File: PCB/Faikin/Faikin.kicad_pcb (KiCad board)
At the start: 2 copper layers, 70 x 70 mm, 27 parts, among them J1 1x5, J2 TC2030-USB-NL-DS, Q1 BSS138PS, U3 MD8942, U4 ESP32-S3-MINI-1

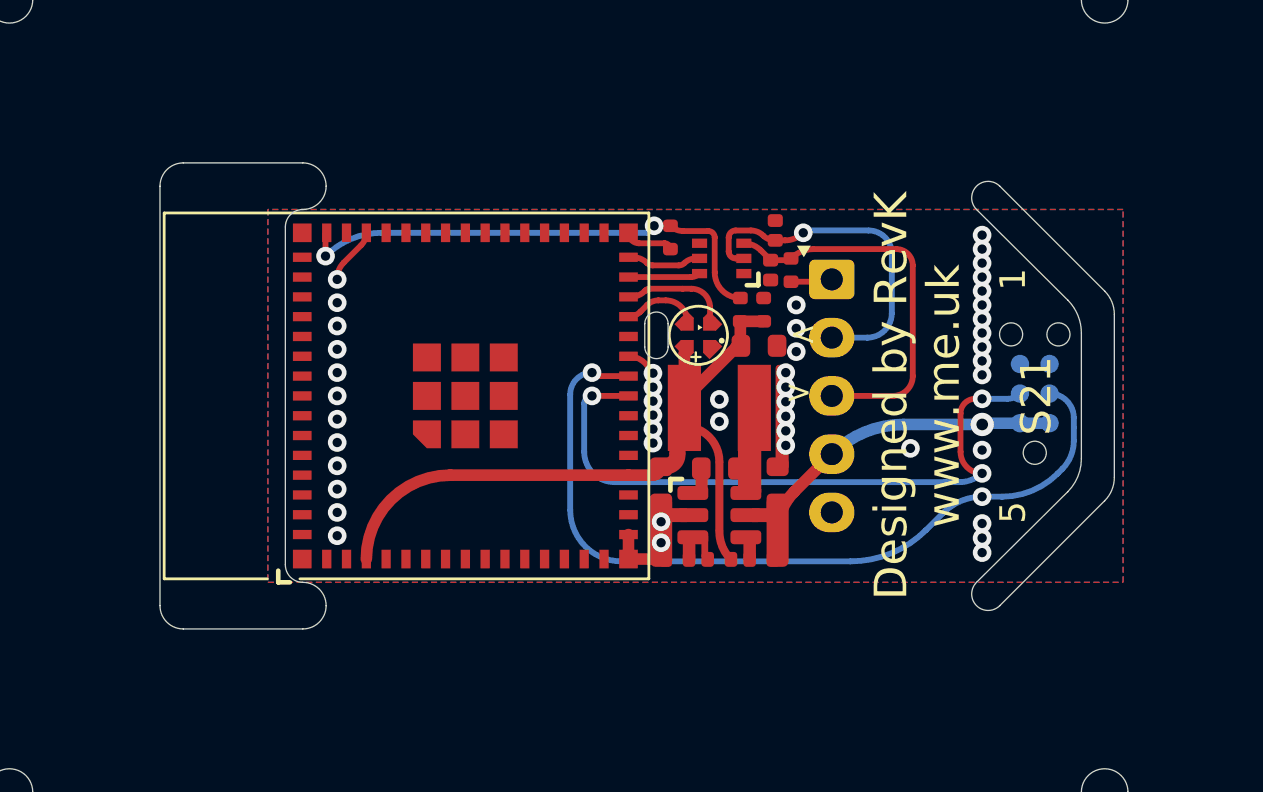
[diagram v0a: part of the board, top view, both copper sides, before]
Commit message: Origin
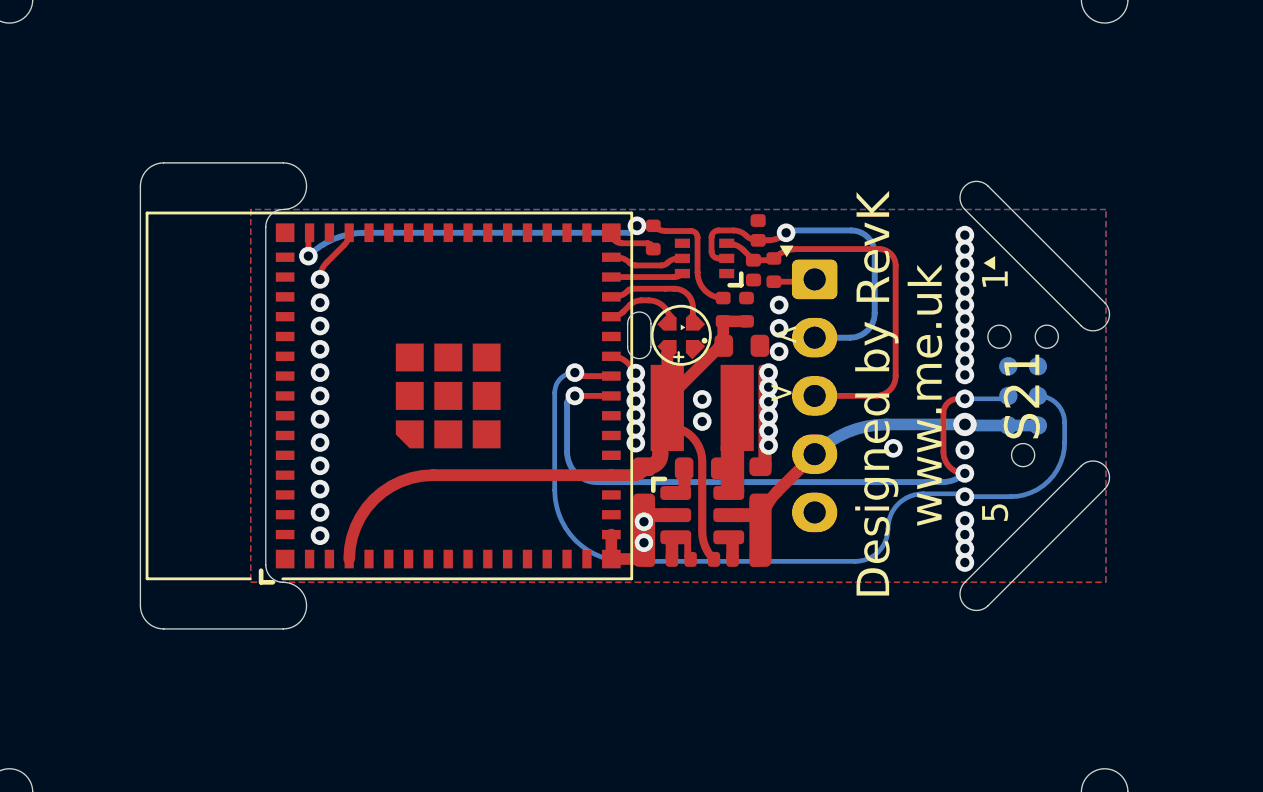
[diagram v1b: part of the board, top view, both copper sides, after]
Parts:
- moved C10 0.74 mm to (140.7, 68.1)
- moved C2 0.74 mm to (142.6, 61.3)
- moved C6 0.74 mm to (138.6, 58.2)
- moved C8 0.74 mm to (143.2, 68.8)
- moved C9 0.74 mm to (138.2, 68.8)
- moved D3 0.74 mm to (143.1, 57.9)
- moved L2 0.74 mm to (140.7, 65.5)
- moved R3 0.74 mm to (141.6, 61.3)
- moved R9 0.74 mm to (140.7, 72.0)
- moved U3 0.74 mm to (140.7, 70.1)
- moved C5 0.73 mm to (142.4, 62.9)
- moved D1 0.73 mm to (139.8, 62.4)
- moved D2 0.73 mm to (142.9, 59.6)
- moved J1 0.73 mm to (145.6, 60.0)
- moved Q1 0.73 mm to (140.8, 59.1)
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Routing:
- net D+: track 35.4 -> 36.1 mm
- net GND: vias 47 -> 48
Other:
- board text added: "®"
